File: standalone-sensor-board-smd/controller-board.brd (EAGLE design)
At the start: 51 x 42 mm, 7 parts, among them J1 DCJ0202

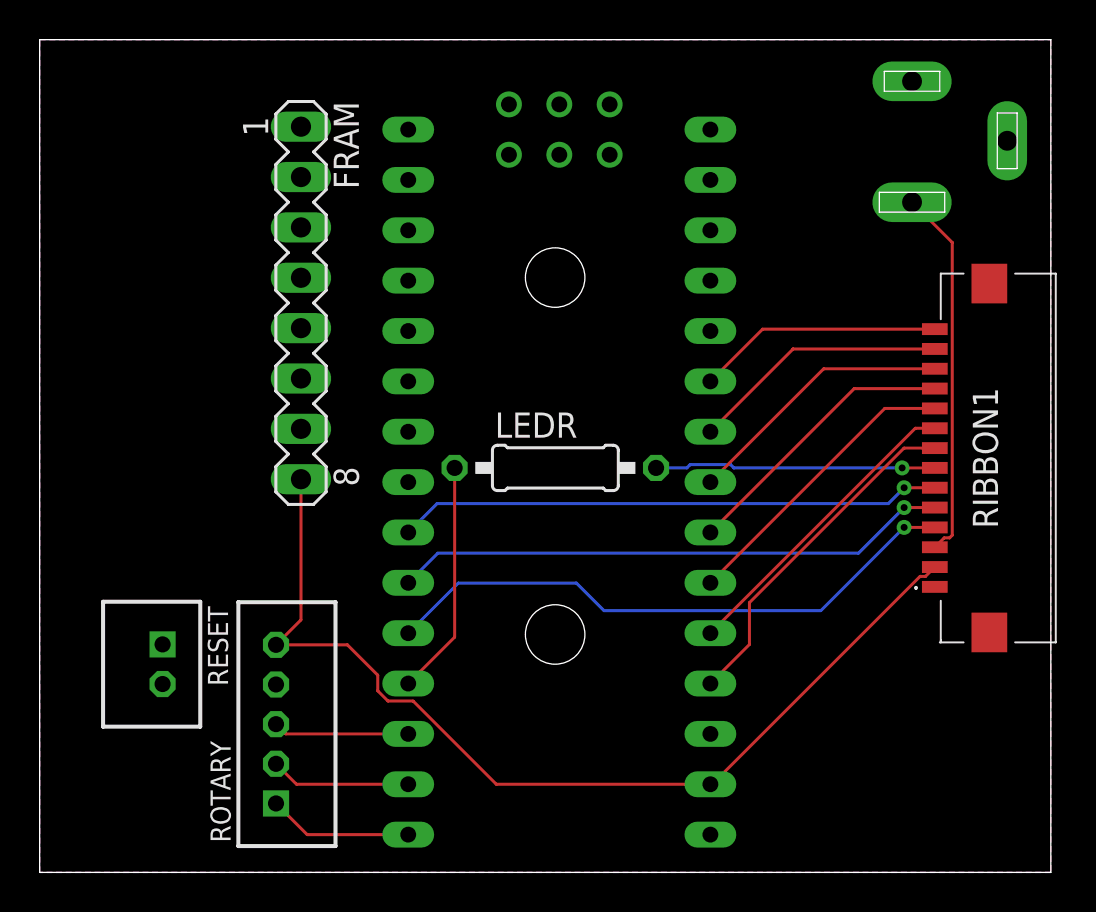
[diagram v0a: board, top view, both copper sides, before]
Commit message: add smd boards from standalone
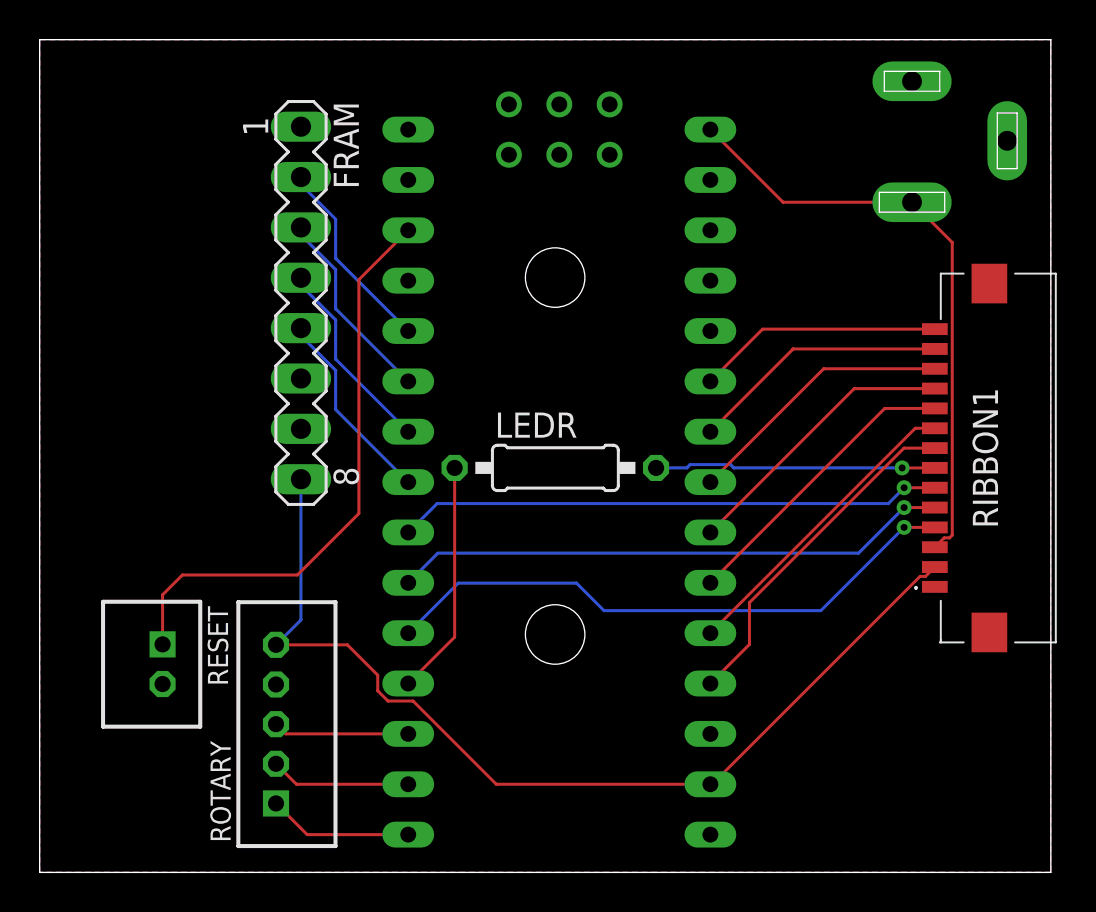
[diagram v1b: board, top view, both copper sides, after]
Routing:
- net RST: track 0.00 -> 29.4 mm
- net VCC: track 18.8 -> 30.5 mm
- net MOSI: track 0.00 -> 10.0 mm
- net MISO: track 0.00 -> 10.0 mm
- net CS: track 0.00 -> 10.0 mm
- net CLK: track 0.00 -> 10.0 mm
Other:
- board text added: "NEMUS Controller Board v0.1.3"
- board text removed: "NEMUS Controller Board v0.1.2"
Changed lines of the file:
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@@
 <rectangle x1="1.995859375" y1="23.867825" x2="8.994859375" y2="23.9225" layer="201"/>
 <rectangle x1="1.995859375" y1="23.813140625" x2="8.994859375" y2="23.867821875" layer="201"/>
-<text x="31.2769625" y="1.96848125" size="0.5" layer="26" font="vector" rot="MR0">NEMUS Controller Board v0.1.2</text>
+<text x="31.2769625" y="1.96848125" size="0.5" layer="26" font="vector" rot="MR0">NEMUS Controller Board v0.1.3</text>
 <hole x="26" y="30" drill="3"/>
 <hole x="26" y="12" drill="3"/>
@@
 <contactref element="U$1" pad="RST1"/>
 <contactref element="RESET" pad="1"/>
-<wire x1="6.2" y1="11.5" x2="18.589" y2="32.385" width="0" layer="19" extent="1-1"/>
+<wire x1="6.2" y1="14" x2="6.2" y2="11.5" width="0.1524" layer="1"/>
+<wire x1="18.589" y1="32.385" x2="16.102" y2="29.898" width="0.1524" layer="1"/>
+<wire x1="16.102" y1="29.898" x2="16.102" y2="18.102" width="0.1524" layer="1"/>
+<wire x1="7.2" y1="15" x2="6.2" y2="14" width="0.1524" layer="1"/>
+<wire x1="16.102" y1="18.102" x2="13" y2="15" width="0.1524" layer="1"/>
+<wire x1="13" y1="15" x2="7.2" y2="15" width="0.1524" layer="1"/>
 </signal>
 <signal name="GND">
@@
 <contactref element="U$1" pad="D2"/>
 <contactref element="FRAM" pad="2"/>
-<wire x1="18.589" y1="27.305" x2="13.18" y2="35.07" width="0" layer="19" extent="1-1"/>
+<wire x1="18.589" y1="27.305" x2="14.9326" y2="30.9614" width="0.1524" layer="16"/>
+<wire x1="13.18" y1="34.692925" x2="13.18" y2="35.07" width="0.1524" layer="16"/>
+<wire x1="14.9326" y1="30.9614" x2="14.9326" y2="32.940325" width="0.1524" layer="16"/>
+<wire x1="14.9326" y1="32.940325" x2="13.18" y2="34.692925" width="0.1524" layer="16"/>
 </signal>
 <signal name="MOSI">
 <contactref element="U$1" pad="D3"/>
 <contactref element="FRAM" pad="3"/>
-<wire x1="18.589" y1="24.765" x2="13.18" y2="32.53" width="0" layer="19" extent="1-1"/>
+<wire x1="18.589" y1="24.765" x2="14.9326" y2="28.4214" width="0.1524" layer="16"/>
+<wire x1="13.18" y1="32.152925" x2="13.18" y2="32.53" width="0.1524" layer="16"/>
+<wire x1="14.9326" y1="28.4214" x2="14.9326" y2="30.400325" width="0.1524" layer="16"/>
+<wire x1="14.9326" y1="30.400325" x2="13.18" y2="32.152925" width="0.1524" layer="16"/>
 </signal>
 <signal name="DIN">
@@
 <wire x1="46.0286" y1="17.0053125" x2="46.0286" y2="31.7714" width="0.1524" layer="1"/>
 <wire x1="46.0286" y1="31.7714" x2="44" y2="33.8" width="0.1524" layer="1"/>
-<wire x1="44" y1="33.8" x2="33.829" y2="37.465" width="0" layer="19" extent="1-1"/>
+<wire x1="44" y1="33.8" x2="37.494" y2="33.8" width="0.1524" layer="1"/>
+<wire x1="37.494" y1="33.8" x2="33.829" y2="37.465" width="0.1524" layer="1"/>
 </signal>
 <signal name="3V">
@@
 <wire x1="23.0311875" y1="4.445" x2="18.8337875" y2="8.6424" width="0.1524" layer="1"/>
 <wire x1="18.8337875" y1="8.6424" x2="17.5694125" y2="8.6424" width="0.1524" layer="1"/>
+<wire x1="17.0524" y1="9.9476" x2="15.523" y2="11.477" width="0.1524" layer="1"/>
 <wire x1="15.523" y1="11.477" x2="11.921" y2="11.477" width="0.1524" layer="1"/>
-<wire x1="17.0524" y1="9.9476" x2="15.523" y2="11.477" width="0.1524" layer="1"/>
-<wire x1="11.921" y1="11.477" x2="13.18" y2="12.736" width="0.1524" layer="1"/>
-<wire x1="13.18" y1="12.736" x2="13.18" y2="19.83" width="0.1524" layer="1"/>
+<wire x1="11.921" y1="11.477" x2="13.18" y2="12.736" width="0.1524" layer="16"/>
+<wire x1="13.18" y1="12.736" x2="13.18" y2="19.83" width="0.1524" layer="16"/>
 </signal>
 <signal name="CLK">
 <contactref element="U$1" pad="D5"/>
 <contactref element="FRAM" pad="5"/>
-<wire x1="18.589" y1="19.685" x2="13.18" y2="27.45" width="0" layer="19" extent="1-1"/>
+<wire x1="18.589" y1="19.685" x2="14.9326" y2="23.3414" width="0.1524" layer="16"/>
+<wire x1="13.18" y1="27.072925" x2="13.18" y2="27.45" width="0.1524" layer="16"/>
+<wire x1="14.9326" y1="23.3414" x2="14.9326" y2="25.320325" width="0.1524" layer="16"/>
+<wire x1="14.9326" y1="25.320325" x2="13.18" y2="27.072925" width="0.1524" layer="16"/>
 </signal>
 <signal name="MISO">
 <contactref element="U$1" pad="D4"/>
 <contactref element="FRAM" pad="4"/>
-<wire x1="18.589" y1="22.225" x2="13.18" y2="29.99" width="0" layer="19" extent="1-1"/>
+<wire x1="18.589" y1="22.225" x2="14.9326" y2="25.8814" width="0.1524" layer="16"/>
+<wire x1="13.18" y1="29.612925" x2="13.18" y2="29.99" width="0.1524" layer="16"/>
+<wire x1="14.9326" y1="25.8814" x2="14.9326" y2="27.860325" width="0.1524" layer="16"/>
+<wire x1="14.9326" y1="27.860325" x2="13.18" y2="29.612925" width="0.1524" layer="16"/>
 </signal>
 <signal name="D9">

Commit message: init smd version
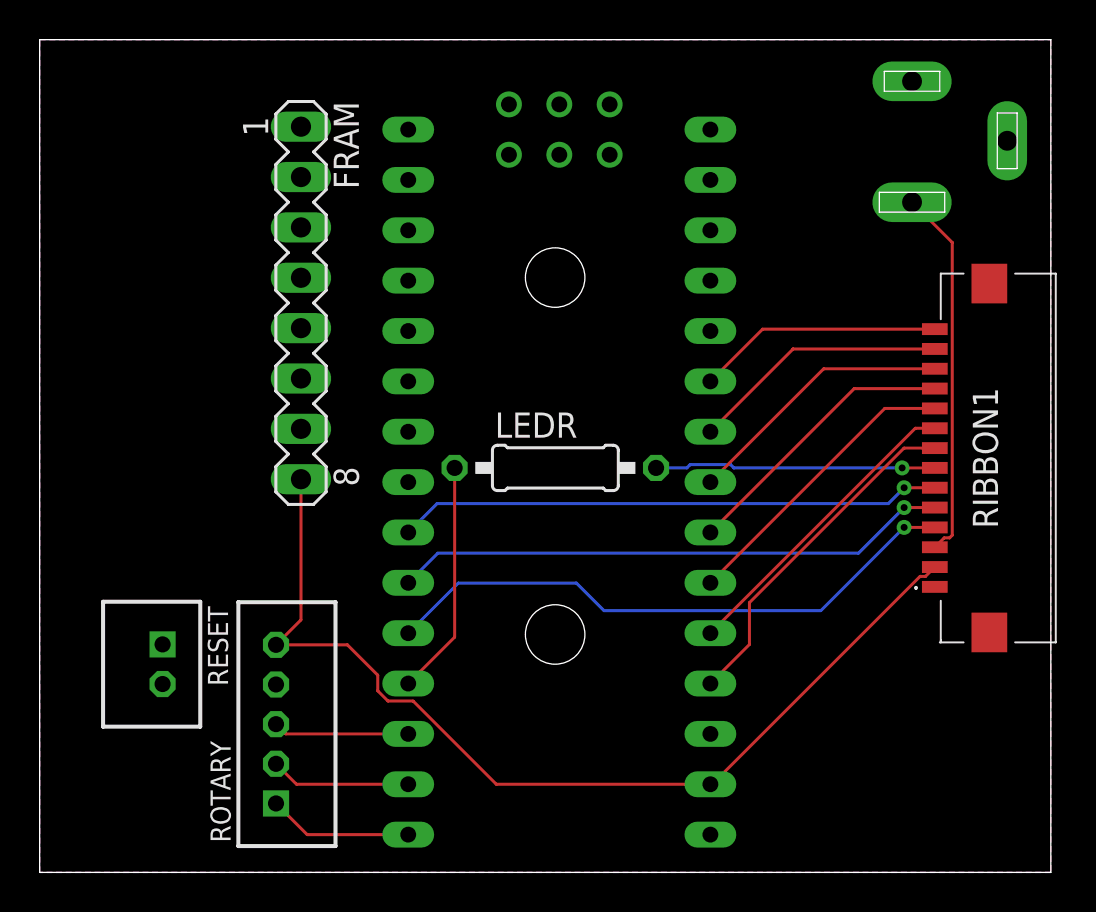
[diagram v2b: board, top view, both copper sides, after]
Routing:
- net RST: track 29.4 -> 0.00 mm
- net VCC: track 30.5 -> 18.8 mm
- net MOSI: track 10.0 -> 0.00 mm
- net MISO: track 10.0 -> 0.00 mm
- net CS: track 10.0 -> 0.00 mm
- net CLK: track 10.0 -> 0.00 mm
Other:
- board text added: "NEMUS Controller Board v0.1.2"
- board text removed: "NEMUS Controller Board v0.1.3"
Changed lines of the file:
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@@
 <rectangle x1="1.995859375" y1="23.867825" x2="8.994859375" y2="23.9225" layer="201"/>
 <rectangle x1="1.995859375" y1="23.813140625" x2="8.994859375" y2="23.867821875" layer="201"/>
-<text x="31.2769625" y="1.96848125" size="0.5" layer="26" font="vector" rot="MR0">NEMUS Controller Board v0.1.3</text>
+<text x="31.2769625" y="1.96848125" size="0.5" layer="26" font="vector" rot="MR0">NEMUS Controller Board v0.1.2</text>
 <hole x="26" y="30" drill="3"/>
 <hole x="26" y="12" drill="3"/>
@@
 <contactref element="U$1" pad="RST1"/>
 <contactref element="RESET" pad="1"/>
-<wire x1="6.2" y1="14" x2="6.2" y2="11.5" width="0.1524" layer="1"/>
-<wire x1="18.589" y1="32.385" x2="16.102" y2="29.898" width="0.1524" layer="1"/>
-<wire x1="16.102" y1="29.898" x2="16.102" y2="18.102" width="0.1524" layer="1"/>
-<wire x1="7.2" y1="15" x2="6.2" y2="14" width="0.1524" layer="1"/>
-<wire x1="16.102" y1="18.102" x2="13" y2="15" width="0.1524" layer="1"/>
-<wire x1="13" y1="15" x2="7.2" y2="15" width="0.1524" layer="1"/>
+<wire x1="6.2" y1="11.5" x2="18.589" y2="32.385" width="0" layer="19" extent="1-1"/>
 </signal>
 <signal name="GND">
@@
 <contactref element="U$1" pad="D2"/>
 <contactref element="FRAM" pad="2"/>
-<wire x1="18.589" y1="27.305" x2="14.9326" y2="30.9614" width="0.1524" layer="16"/>
-<wire x1="13.18" y1="34.692925" x2="13.18" y2="35.07" width="0.1524" layer="16"/>
-<wire x1="14.9326" y1="30.9614" x2="14.9326" y2="32.940325" width="0.1524" layer="16"/>
-<wire x1="14.9326" y1="32.940325" x2="13.18" y2="34.692925" width="0.1524" layer="16"/>
+<wire x1="18.589" y1="27.305" x2="13.18" y2="35.07" width="0" layer="19" extent="1-1"/>
 </signal>
 <signal name="MOSI">
 <contactref element="U$1" pad="D3"/>
 <contactref element="FRAM" pad="3"/>
-<wire x1="18.589" y1="24.765" x2="14.9326" y2="28.4214" width="0.1524" layer="16"/>
-<wire x1="13.18" y1="32.152925" x2="13.18" y2="32.53" width="0.1524" layer="16"/>
-<wire x1="14.9326" y1="28.4214" x2="14.9326" y2="30.400325" width="0.1524" layer="16"/>
-<wire x1="14.9326" y1="30.400325" x2="13.18" y2="32.152925" width="0.1524" layer="16"/>
+<wire x1="18.589" y1="24.765" x2="13.18" y2="32.53" width="0" layer="19" extent="1-1"/>
 </signal>
 <signal name="DIN">
@@
 <wire x1="46.0286" y1="17.0053125" x2="46.0286" y2="31.7714" width="0.1524" layer="1"/>
 <wire x1="46.0286" y1="31.7714" x2="44" y2="33.8" width="0.1524" layer="1"/>
-<wire x1="44" y1="33.8" x2="37.494" y2="33.8" width="0.1524" layer="1"/>
-<wire x1="37.494" y1="33.8" x2="33.829" y2="37.465" width="0.1524" layer="1"/>
+<wire x1="44" y1="33.8" x2="33.829" y2="37.465" width="0" layer="19" extent="1-1"/>
 </signal>
 <signal name="3V">
@@
 <wire x1="23.0311875" y1="4.445" x2="18.8337875" y2="8.6424" width="0.1524" layer="1"/>
 <wire x1="18.8337875" y1="8.6424" x2="17.5694125" y2="8.6424" width="0.1524" layer="1"/>
+<wire x1="15.523" y1="11.477" x2="11.921" y2="11.477" width="0.1524" layer="1"/>
 <wire x1="17.0524" y1="9.9476" x2="15.523" y2="11.477" width="0.1524" layer="1"/>
-<wire x1="15.523" y1="11.477" x2="11.921" y2="11.477" width="0.1524" layer="1"/>
-<wire x1="11.921" y1="11.477" x2="13.18" y2="12.736" width="0.1524" layer="16"/>
-<wire x1="13.18" y1="12.736" x2="13.18" y2="19.83" width="0.1524" layer="16"/>
+<wire x1="11.921" y1="11.477" x2="13.18" y2="12.736" width="0.1524" layer="1"/>
+<wire x1="13.18" y1="12.736" x2="13.18" y2="19.83" width="0.1524" layer="1"/>
 </signal>
 <signal name="CLK">
 <contactref element="U$1" pad="D5"/>
 <contactref element="FRAM" pad="5"/>
-<wire x1="18.589" y1="19.685" x2="14.9326" y2="23.3414" width="0.1524" layer="16"/>
-<wire x1="13.18" y1="27.072925" x2="13.18" y2="27.45" width="0.1524" layer="16"/>
-<wire x1="14.9326" y1="23.3414" x2="14.9326" y2="25.320325" width="0.1524" layer="16"/>
-<wire x1="14.9326" y1="25.320325" x2="13.18" y2="27.072925" width="0.1524" layer="16"/>
+<wire x1="18.589" y1="19.685" x2="13.18" y2="27.45" width="0" layer="19" extent="1-1"/>
 </signal>
 <signal name="MISO">
 <contactref element="U$1" pad="D4"/>
 <contactref element="FRAM" pad="4"/>
-<wire x1="18.589" y1="22.225" x2="14.9326" y2="25.8814" width="0.1524" layer="16"/>
-<wire x1="13.18" y1="29.612925" x2="13.18" y2="29.99" width="0.1524" layer="16"/>
-<wire x1="14.9326" y1="25.8814" x2="14.9326" y2="27.860325" width="0.1524" layer="16"/>
-<wire x1="14.9326" y1="27.860325" x2="13.18" y2="29.612925" width="0.1524" layer="16"/>
+<wire x1="18.589" y1="22.225" x2="13.18" y2="29.99" width="0" layer="19" extent="1-1"/>
 </signal>
 <signal name="D9">
